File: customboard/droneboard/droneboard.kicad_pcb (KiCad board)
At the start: 4 copper layers, 38 x 38 mm, 49 parts, among them J1 Conn_01x04, J3 Conn_01x05_Pin, J4 Conn_01x02_Pin, J7 Conn_01x04_Odd_Even, SW1 SW_Push, SW2 SW_Push, U1 STM32F411CEUx, U3 L78M05CDT, U4 ICM-42688-P, U5 LDK130M33R, U6 LDK130M33R, Y2 CSTNE20M0V53Z000R0

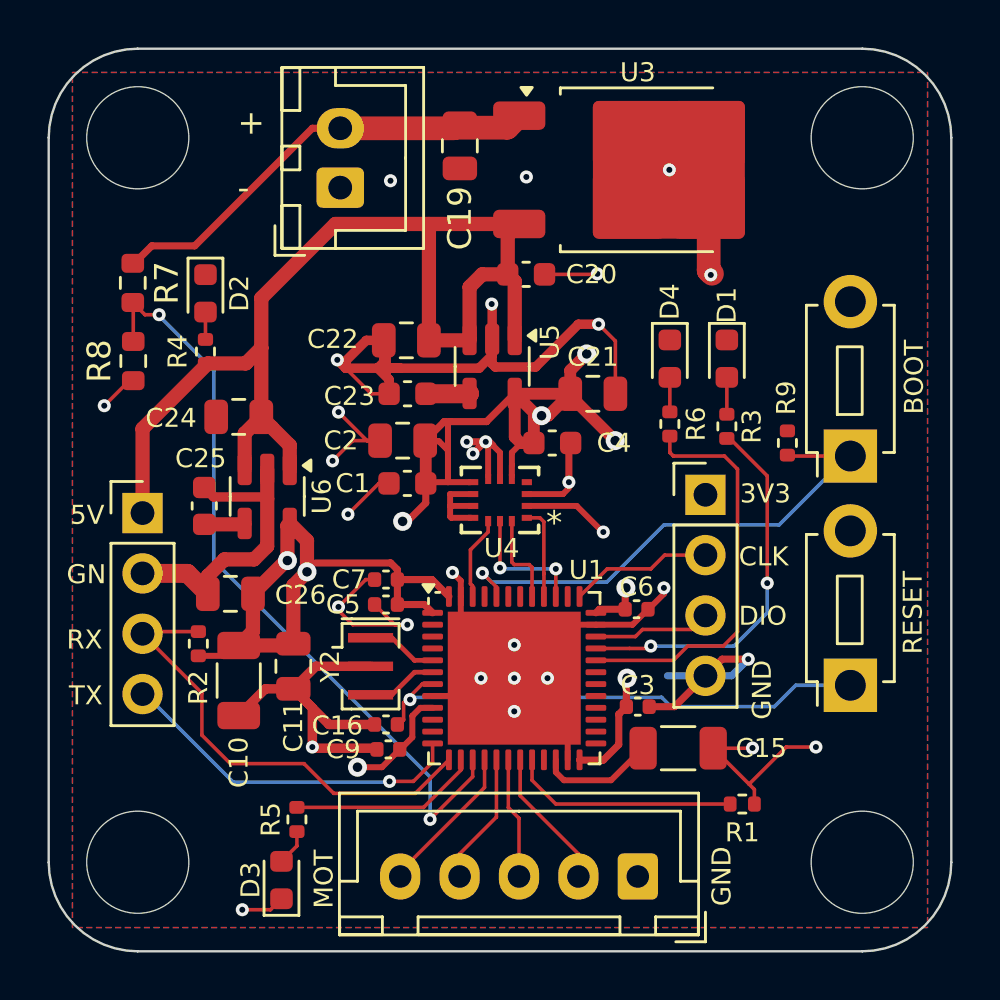
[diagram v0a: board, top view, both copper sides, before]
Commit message: usb implementation start
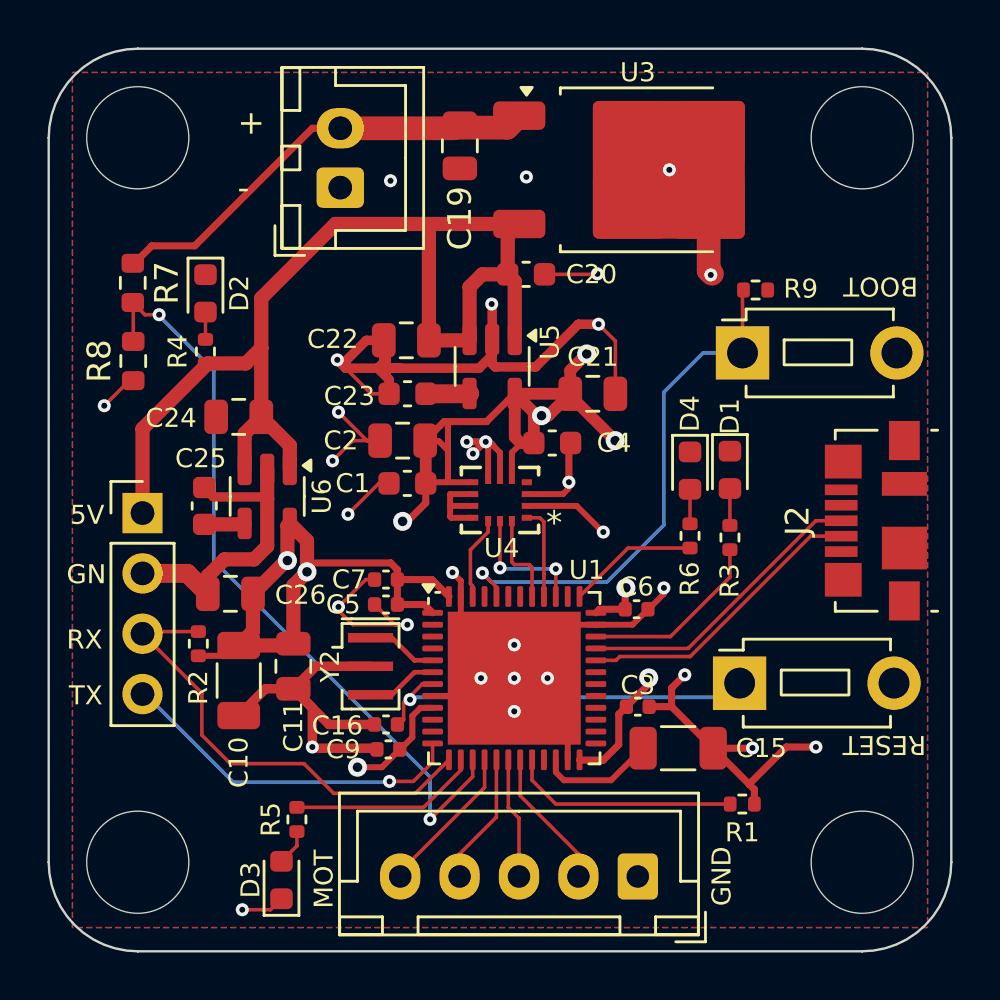
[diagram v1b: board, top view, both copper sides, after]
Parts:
- removed J7: Conn_01x04_Odd_Even, Connector_PinHeader_2.54mm:PinHeader_1x04_P2.54mm_Vertical
- added J2: USB_B_Micro, Connector_USB:USB_Micro-B_Molex_47346-0001, F.Cu at (84.8, 101.9)
- moved R9 6.58 mm to (79.8, 92.2), turned to 180 degrees
- moved SW2 6.28 mm to (79.2, 94.8), turned to 0 degrees
- moved D4 4.79 mm to (77.0, 99.8)
- moved R6 4.79 mm to (77.0, 102.5)
- moved D1 4.68 mm to (78.7, 99.7)
- moved R3 4.68 mm to (78.7, 102.6)
- moved SW1 4.66 mm to (79.1, 108.7), turned to 0 degrees
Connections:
- U1 pad 32: /BLUE -> /USB_DM
- U1 pad 33: /YELLOW -> /USB_DP
- U1 pad 34: /SWDIO -> /YELLOW
- U1 pad 37: /SWCLK -> /BLUE
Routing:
- net /USB_DP: track 0.00 -> 12.6 mm
- net /USB_DM: track 0.00 -> 12.5 mm
- net /BLUE: track 17.1 -> 5.49 mm
- net /YELLOW: track 16.0 -> 7.84 mm, vias 2 -> 0
- net /SWCLK: track 6.02 -> 0.00 mm
- net /SWDIO: track 4.98 -> 0.00 mm
- net /RESET1: track 21.9 -> 16.9 mm
- net /GND: track 134.7 -> 131.0 mm
- net /BOOT: track 21.8 -> 22.4 mm
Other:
- board text removed: "3V3"
- board text removed: "CLK"
- board text removed: "DIO"
